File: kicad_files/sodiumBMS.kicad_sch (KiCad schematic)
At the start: 39 parts, among them J1 USB_C_Receptacle_PowerOnly_6P, Q1 AO3400A, Q2 AO3400A, U1 STM32F446RETx, U2 INA180A4, U3 INA180A4, U4 LM3940, U5 MC34063AD

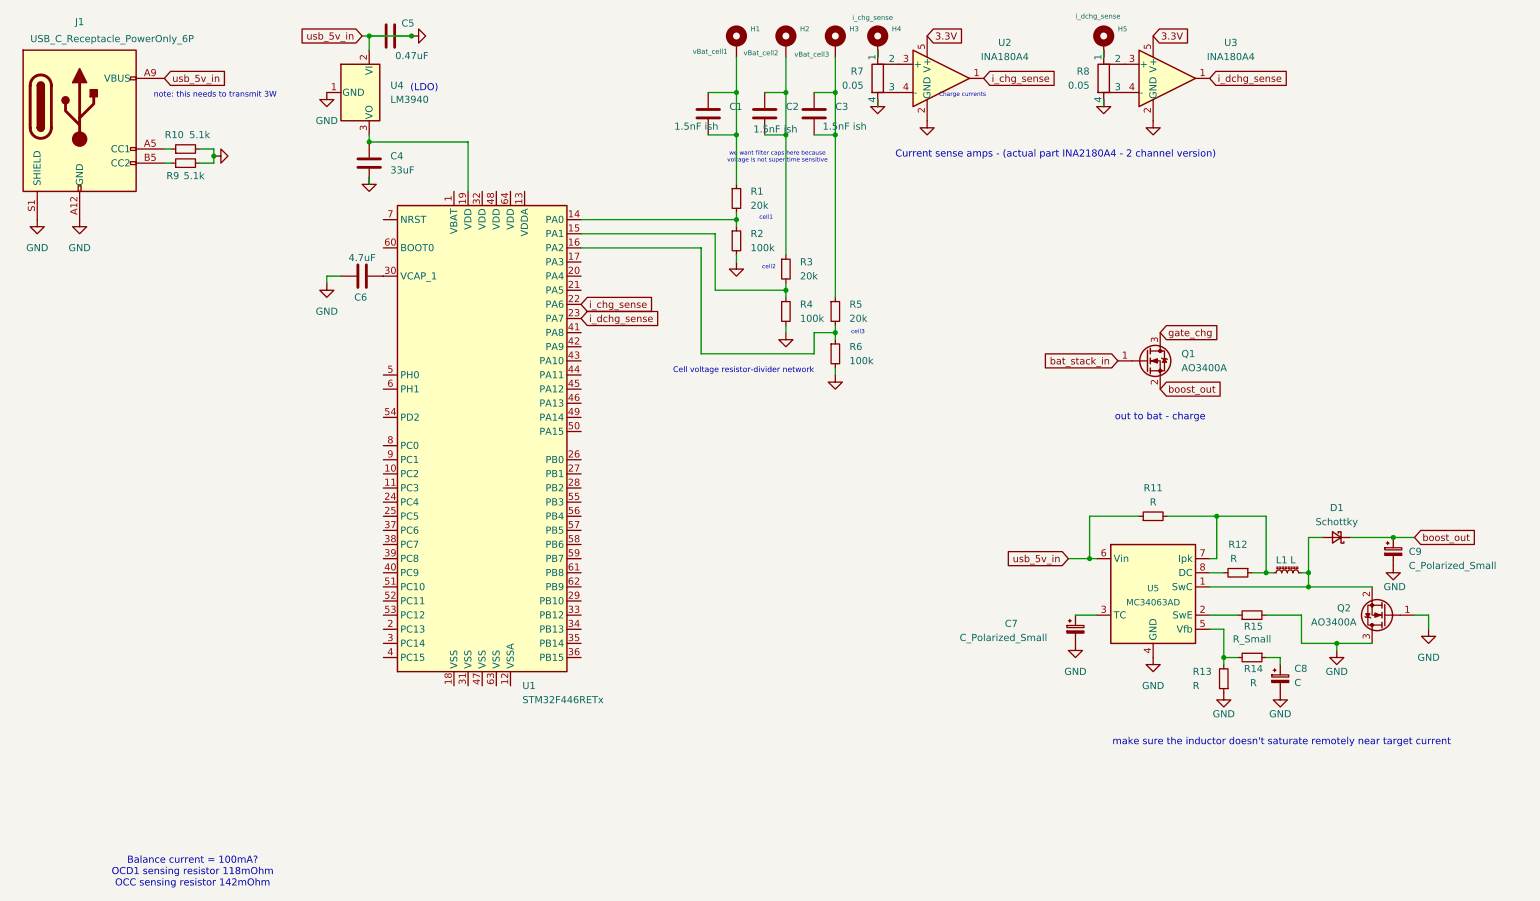
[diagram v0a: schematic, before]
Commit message: separate sheets now, pretty much done with schematic just gotta do some documentation
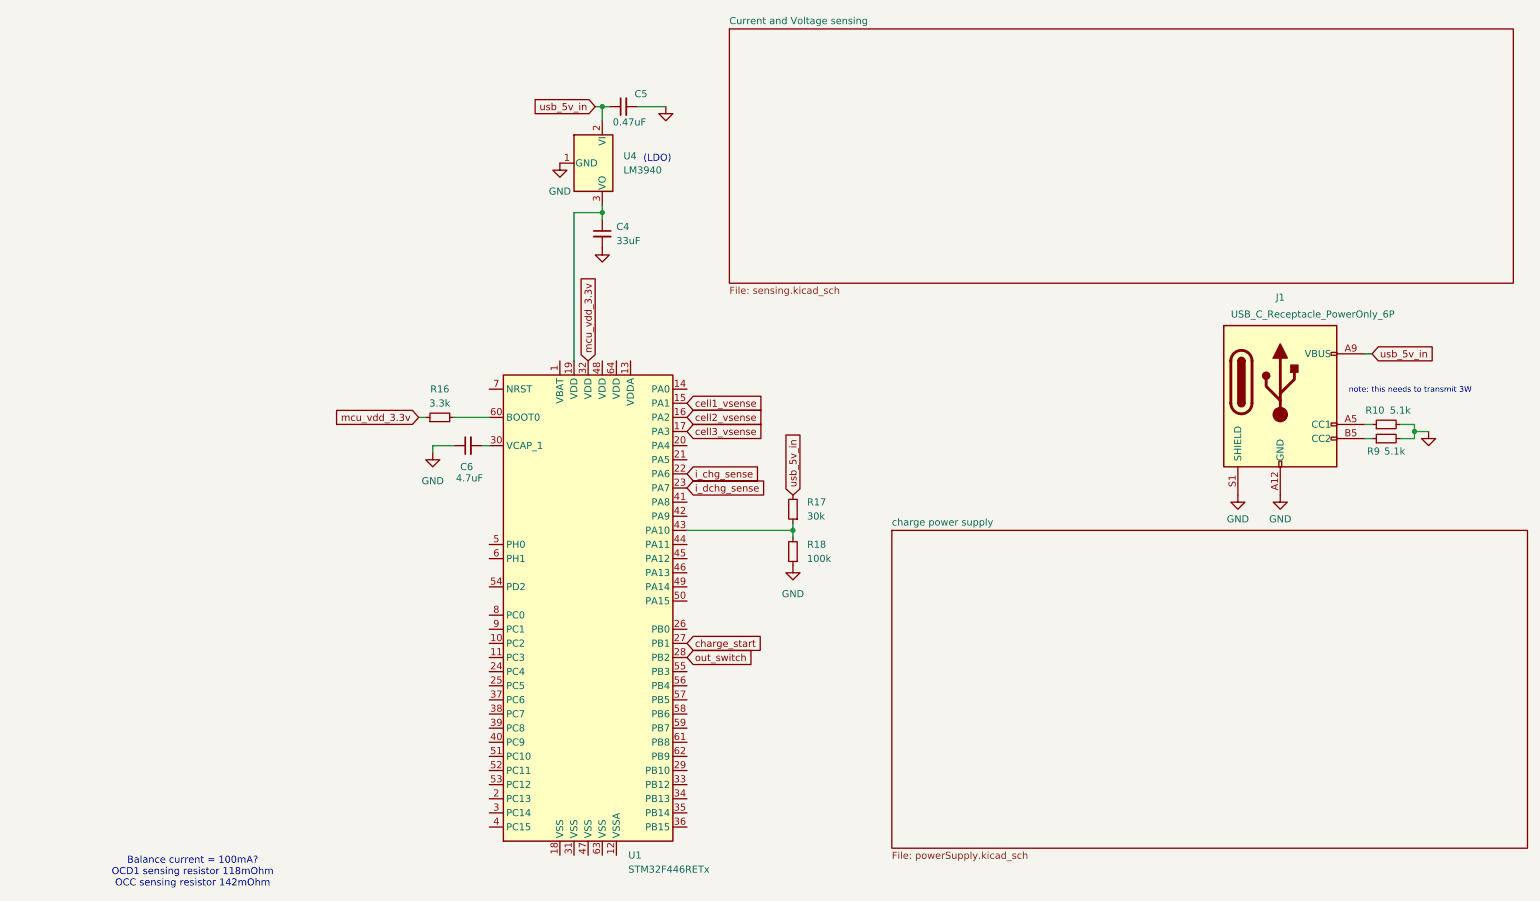
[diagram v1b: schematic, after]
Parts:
- removed C1, C2, C3: 1.5nF ish, symbol Device:C
- removed C7, C9: C_Polarized_Small, symbol Device:C_Polarized_Small
- removed C8: C, symbol Device:C_Polarized_Small
- removed D1: Schottky, symbol Device:D_Schottky_Small
- removed H1: vBat_cell1, symbol Mechanical:MountingHole_Pad
- removed H2: vBat_cell2, symbol Mechanical:MountingHole_Pad
- removed H3: vBat_cell3, symbol Mechanical:MountingHole_Pad
- removed H4: i_chg_sense, symbol Mechanical:MountingHole_Pad
- removed H5: i_dchg_sense, symbol Mechanical:MountingHole_Pad
- removed L1: L, symbol Device:L_Ferrite_Small
- removed Q1, Q2: AO3400A, Package_TO_SOT_SMD:SOT-23, symbol Transistor_FET:AO3400A
- removed R1, R3, R5: 20k, symbol Device:R_Small
- removed R11, R12, R13, R14: R, symbol Device:R_Small
- removed R15: R_Small, symbol Device:R_Small
- removed R2, R4, R6: 100k, symbol Device:R_Small
- removed R7, R8: 0.05, symbol Device:R_Shunt
- removed U2, U3: INA180A4, Package_TO_SOT_SMD:SOT-23-5, symbol Amplifier_Current:INA180A4
- removed U5: MC34063AD, Package_SO:SOIC-8_3.9x4.9mm_P1.27mm, symbol Regulator_Switching:MC34063AD
- added R16: 3.3k, symbol Device:R_Small
- added R17: 30k, symbol Device:R_Small
- added R18: 100k, symbol Device:R_Small
- C4, C5, C6: symbol Device:C -> Device:C_Small
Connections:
- net GND: now also R18.1; no longer C5.1, J1.A9 (VBUS), J1.B9 (VBUS), U4.2 (VI)
- net cell2_vsense: now reaches U1.16 (PA2)
- net cell1_vsense: now reaches U1.15 (PA1)
- net cell3_vsense: now reaches U1.17 (PA3)
- net charge_start: now reaches U1.27 (PB1)
- net out_switch: now reaches U1.28 (PB2)
- net mcu_vdd_3.3v: now reaches U1.32 (VDD)
- net mcu_vdd_3.3v: now also R16.1
- net at U1.43 (PA10): now also R17.1, R18.2
- net at U1.60 (BOOT0): now also R16.2
- new net usb_5v_in: C5.1, J1.A9 (VBUS), J1.B9 (VBUS), R17.2, U4.2 (VI)
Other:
- added sheet Current and Voltage sensing (sensing.kicad_sch)
- added sheet charge power supply (powerSupply.kicad_sch)
- note removed: "Cell voltage resistor-divider network"
- note removed: "Charge currents"
- note removed: "Current sense amps - (actual part INA2180A4 - 2 channel version)"
- note removed: "cell1"
- note removed: "cell2"
- note removed: "cell3"
- note removed: "make sure the inductor doesn't saturate remotely near target current"
- note removed: "out to bat - charge"
- note removed: "we want filter caps here because voltage is not super time sensitive"
- moved on the sheet: C4, C5, C6, J1, R10, R9, U1, U4
